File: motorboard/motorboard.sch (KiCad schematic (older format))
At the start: 29 parts

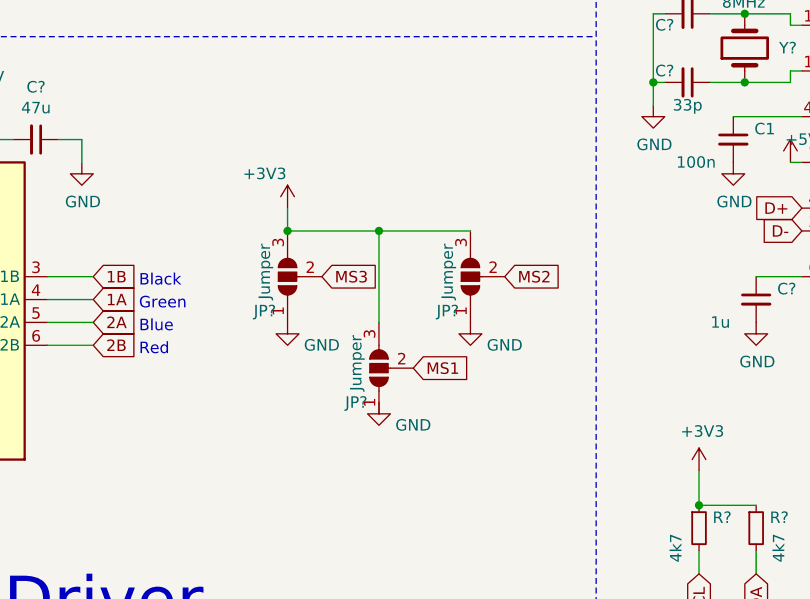
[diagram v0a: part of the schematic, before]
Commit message: tidying things
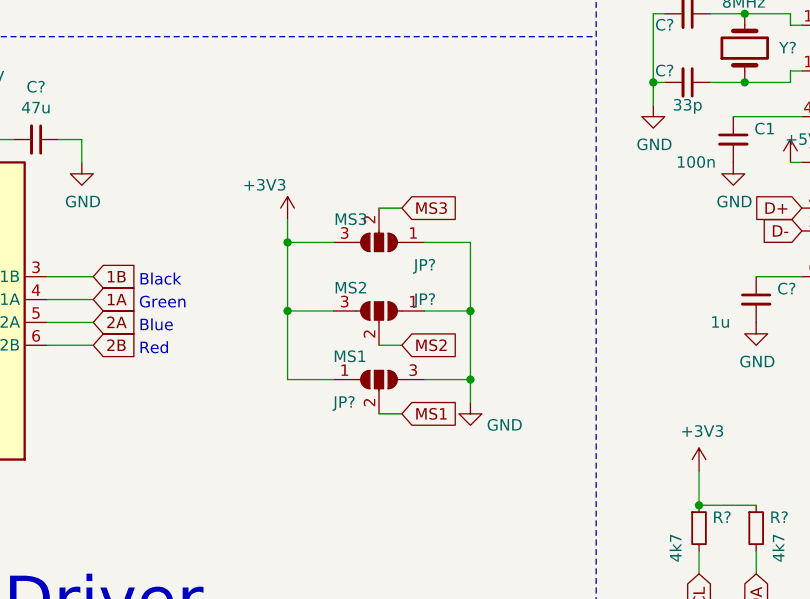
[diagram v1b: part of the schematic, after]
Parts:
- removed JP? (x3): Jumper, symbol Jumper:SolderJumper_3_Open
- added JP?: MS1, symbol Jumper:SolderJumper_3_Open
- added JP?: MS3, symbol Jumper:SolderJumper_3_Open
- added JP?: MS2, symbol Jumper:SolderJumper_3_Open
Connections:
- wire segments 130 -> 141
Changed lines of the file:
@@
 Text Notes 5800 3000 0    50   ~ 0
 Red
-$Comp
-L power:+3V3 #PWR?
-U 1 1 5E52FFC7
-P 6450 2350
-F 0 "#PWR?" H 6450 2200 50  0001 C CNN
-F 1 "+3V3" H 6350 2500 50  0000 C CNN
-F 2 "" H 6450 2350 50  0001 C CNN
-F 3 "" H 6450 2350 50  0001 C CNN
-	1    6450 2350
-	1    0    0    -1
-$EndComp
 Wire Wire Line
 	4500 2450 4400 2450
@@
 Text Notes 4000 6000 0    207  ~ 0
 Connectors
-$Comp
-L Device:Crystal Y?
-U 1 1 5E5C2710
-P 8450 1650
-F 0 "Y?" V 8450 1500 50  0000 R CNN
-F 1 "8MHz" V 8650 1750 50  0000 R CNN
-F 2 "" H 8450 1650 50  0001 C CNN
-F 3 "~" H 8450 1650 50  0001 C CNN
-	1    8450 1650
-	0    -1   -1   0
-$EndComp
 Wire Wire Line
 	8700 1550 8650 1550
@@
 	8650 1550 8650 1500
 Wire Wire Line
-	8650 1500 8450 1500
-Wire Wire Line
 	8700 1750 8650 1750
 Wire Wire Line
 	8650 1750 8650 1800
-Wire Wire Line
-	8650 1800 8450 1800
 $Comp
 L power:GND #PWR?
@@
 	0    1    1    0
 $EndComp
-Wire Wire Line
-	8450 1500 8300 1500
-Connection ~ 8450 1500
-Wire Wire Line
-	8450 1800 8300 1800
-Connection ~ 8450 1800
 Wire Wire Line
 	8100 1800 8050 1800
@@
 	1    0    0    -1
 $EndComp
-$Comp
-L Jumper:SolderJumper_3_Open JP?
-U 1 1 5E72A5E4
-P 7250 2650
-F 0 "JP?" V 7100 2700 50  0000 L CNN
-F 1 "Jumper" H 7150 2750 50  0000 L CNN
-F 2 "" H 7250 2650 50  0001 C CNN
-F 3 "~" H 7250 2650 50  0001 C CNN
-	1    7250 2650
-	0    -1   -1   0
-$EndComp
-$Comp
-L Jumper:SolderJumper_3_Open JP?
-U 1 1 5E72EB25
-P 6450 2650
-F 0 "JP?" V 6300 2700 50  0000 L CNN
-F 1 "Jumper" H 6350 2750 50  0000 L CNN
-F 2 "" H 6450 2650 50  0001 C CNN
-F 3 "~" H 6450 2650 50  0001 C CNN
-	1    6450 2650
-	0    -1   -1   0
-$EndComp
 Text GLabel 4500 3050 0    50   Input ~ 0
 MS1
@@
 Text GLabel 4500 3250 0    50   Input ~ 0
 MS3
-$Comp
-L Jumper:SolderJumper_3_Open JP?
-U 1 1 5E736A16
-P 6850 3050
-F 0 "JP?" V 6700 3100 50  0000 L CNN
-F 1 "Jumper" H 6750 3150 50  0000 L CNN
-F 2 "" H 6850 3050 50  0001 C CNN
-F 3 "~" H 6850 3050 50  0001 C CNN
-	1    6850 3050
-	0    -1   -1   0
-$EndComp
-Text GLabel 7000 3050 2    50   Input ~ 0
-MS1
-Text GLabel 7400 2650 2    50   Input ~ 0
-MS2
-Text GLabel 6600 2650 2    50   Input ~ 0
-MS3
-Connection ~ 6850 2450
-Wire Wire Line
-	6850 2850 6850 2450
 $Comp
 L power:+3V3 #PWR?
@@
 Wire Wire Line
 	10850 2400 10850 2300
-Wire Wire Line
-	6450 2450 6850 2450
-Wire Wire Line
-	6850 2450 7250 2450
-$Comp
-L power:GND #PWR?
-U 1 1 5E7A289F
-P 6450 2850
-F 0 "#PWR?" H 6450 2600 50  0001 C CNN
-F 1 "GND" H 6600 2750 50  0000 C CNN
-F 2 "" H 6450 2850 50  0001 C CNN
-F 3 "" H 6450 2850 50  0001 C CNN
-	1    6450 2850
-	1    0    0    -1
-$EndComp
-$Comp
-L power:GND #PWR?
-U 1 1 5E7A3015
-P 6850 3200
-F 0 "#PWR?" H 6850 2950 50  0001 C CNN
-F 1 "GND" H 7000 3100 50  0000 C CNN
-F 2 "" H 6850 3200 50  0001 C CNN
-F 3 "" H 6850 3200 50  0001 C CNN
-	1    6850 3200
-	1    0    0    -1
-$EndComp
-$Comp
-L power:GND #PWR?
-U 1 1 5E7A32E6
-P 7250 2850
-F 0 "#PWR?" H 7250 2600 50  0001 C CNN
-F 1 "GND" H 7400 2750 50  0000 C CNN
-F 2 "" H 7250 2850 50  0001 C CNN
-F 3 "" H 7250 2850 50  0001 C CNN
-	1    7250 2850
-	1    0    0    -1
-$EndComp
 Wire Wire Line
 	9900 2350 10100 2350
@@
 Wire Wire Line
 	8500 2650 8700 2650
-Wire Wire Line
-	6450 2450 6450 2350
-Connection ~ 6450 2450
+$Comp
+L power:GND #PWR?
+U 1 1 5E8ED772
+P 7250 3200
+F 0 "#PWR?" H 7250 2950 50  0001 C CNN
+F 1 "GND" H 7400 3100 50  0000 C CNN
+F 2 "" H 7250 3200 50  0001 C CNN
+F 3 "" H 7250 3200 50  0001 C CNN
+	1    7250 3200
+	1    0    0    -1
+$EndComp
+Text GLabel 6950 2350 2    50   Input ~ 0
+MS3
+Text GLabel 6950 2950 2    50   Input ~ 0
+MS2
+Text GLabel 6950 3250 2    50   Input ~ 0
+MS1
+$Comp
+L Jumper:SolderJumper_3_Open JP?
+U 1 1 5E8ED785
+P 6850 2500
+F 0 "JP?" H 6600 2600 50  0000 L CNN
+F 1 "MS3" H 6900 2400 50  0000 L CNN
+F 2 "" H 6850 2500 50  0001 C CNN
+F 3 "~" H 6850 2500 50  0001 C CNN
+	1    6850 2500
+	-1   0    0    1
+$EndComp
+$Comp
+L Jumper:SolderJumper_3_Open JP?
+U 1 1 5E8ED78B
+P 6850 2800
+F 0 "JP?" H 6600 2850 50  0000 L CNN
+F 1 "MS2" H 6900 2900 50  0000 L CNN
+F 2 "" H 6850 2800 50  0001 C CNN
+F 3 "~" H 6850 2800 50  0001 C CNN
+	1    6850 2800
+	-1   0    0    -1
+$EndComp
+$Comp
+L power:+3V3 #PWR?
+U 1 1 5E8ED791
+P 6450 2400
+F 0 "#PWR?" H 6450 2250 50  0001 C CNN
+F 1 "+3V3" H 6350 2550 50  0000 C CNN
+F 2 "" H 6450 2400 50  0001 C CNN
+F 3 "" H 6450 2400 50  0001 C CNN
+	1    6450 2400
+	1    0    0    -1
+$EndComp
+$Comp
+L Jumper:SolderJumper_3_Open JP?
+U 1 1 5E8ED77F
+P 6850 3100
+F 0 "JP?" H 6650 3000 50  0000 L CNN
+F 1 "MS1" H 6650 3200 50  0000 L CNN
+F 2 "" H 6850 3100 50  0001 C CNN
+F 3 "~" H 6850 3100 50  0001 C CNN
+	1    6850 3100
+	1    0    0    -1
+$EndComp
+Wire Wire Line
+	7050 3100 7250 3100
+Wire Wire Line
+	7250 3100 7250 3200
+Wire Wire Line
+	7050 2500 7250 2500
+Wire Wire Line
+	7250 2800 7250 3100
+Wire Wire Line
+	7050 2800 7250 2800
+Connection ~ 7250 3100
+Wire Wire Line
+	7250 2800 7250 2500
+Connection ~ 7250 2800
+Wire Wire Line
+	6950 3250 6850 3250
+Wire Wire Line
+	6950 2950 6850 2950
+Wire Wire Line
+	6950 2350 6850 2350
+Wire Wire Line
+	6450 2500 6650 2500
+Wire Wire Line
+	6650 3100 6450 3100
+Connection ~ 6450 2500
+Wire Wire Line
+	6650 2800 6450 2800
+Wire Wire Line
+	6450 2500 6450 2800
+Connection ~ 6450 2800
+Wire Wire Line
+	6450 2800 6450 3100
+Wire Wire Line
+	6450 2400 6450 2500
+Connection ~ 8450 1800
+Connection ~ 8450 1500
+Wire Wire Line
+	8450 1800 8300 1800
+Wire Wire Line
+	8650 1800 8450 1800
+Wire Wire Line
+	8450 1500 8300 1500
+Wire Wire Line
+	8650 1500 8450 1500
+$Comp
+L Device:Crystal Y?
+U 1 1 5E5C2710
+P 8450 1650
+F 0 "Y?" V 8450 1500 50  0000 R CNN
+F 1 "8MHz" V 8650 1750 50  0000 R CNN
+F 2 "" H 8450 1650 50  0001 C CNN
+F 3 "~" H 8450 1650 50  0001 C CNN
+	1    8450 1650
+	0    -1   -1   0
+$EndComp
 $EndSCHEMATC
